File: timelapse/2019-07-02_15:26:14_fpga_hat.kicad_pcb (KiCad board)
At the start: 4 copper layers, 65 x 56.5 mm, 90 parts, among them J1 2x20, J2 AudioJack3, J3 Conn_02x06_Top_Bottom, J4 Conn_02x06_Top_Bottom, J5 Conn_02x06_Top_Bottom, J6 Conn_01x02, SW1 PTS815, SW2 PTS815, SW3 PTS815, SW4 PTS815, SW5 PTS815, SW6 PTS815, SW7 PTS815, SW8 PTS815, SW9 PTS815, U1 iCE40-HX8k-BG121, U2 CAT24C32WI, U3 MIC23050-4YML, U4 74LVC2G07, U5 DSC60XX, U6 NCP115ASN330T, U7 W25X40CL, U8 IS61WV25616

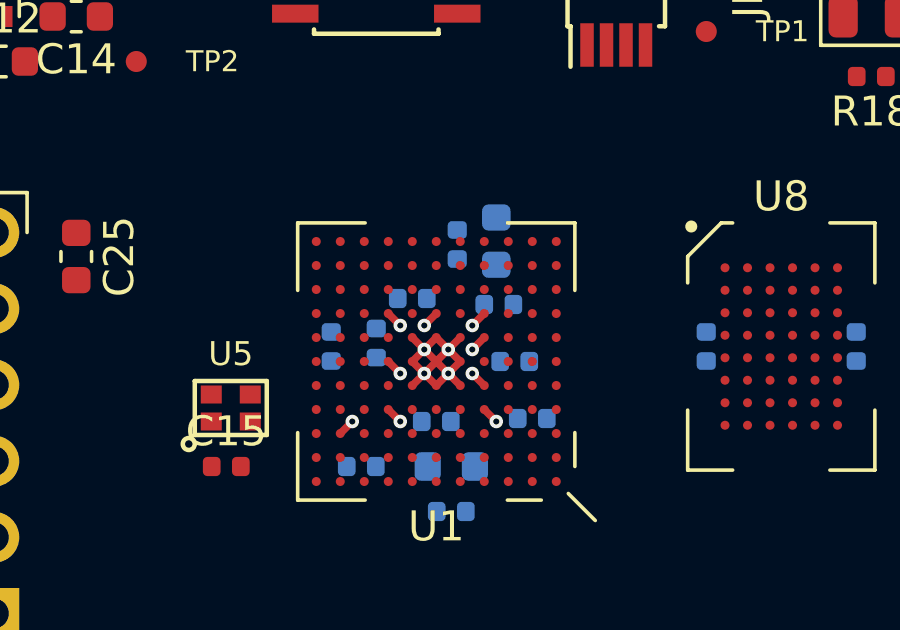
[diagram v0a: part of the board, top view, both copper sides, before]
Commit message: All parts on board
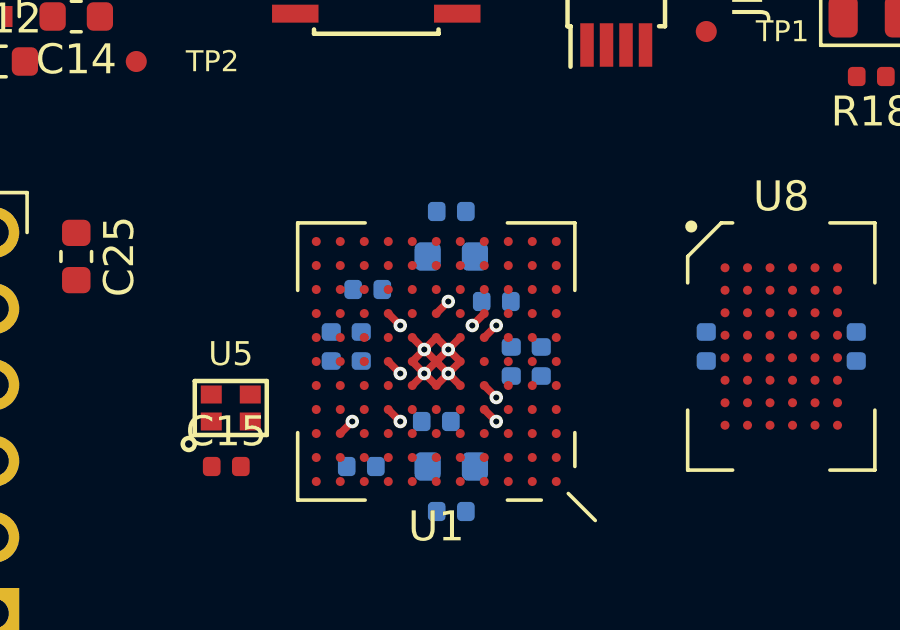
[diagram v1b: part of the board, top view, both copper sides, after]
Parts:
- moved C6 4.40 mm to (130.2, 104.1), turned to 180 degrees
- moved C11 2.80 mm to (134.5, 104.5), turned to 0 degrees
- moved C5 2.02 mm to (135.0, 106.5), turned to 90 degrees
- moved C2 1.59 mm to (133.0, 103.0), turned to 180 degrees
- moved R2 1.12 mm to (133.0, 101.5), turned to 0 degrees
- moved C7 0.88 mm to (136.0, 106.5), turned to 90 degrees
- moved C1 0.51 mm to (130.0, 106.0)
